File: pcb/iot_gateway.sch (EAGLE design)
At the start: 183 parts, among them CON1 6P-SH-TOP, CON2 6P-SH-TOP, CON3 2P-PH-TOP, J2 DCJACK-SMD, Q1 AO3401, Q2 AO3401, Q3 AO3400, Q4 AO3400, T1 BC817, T2 BC817, T3 BC817, T4 BC817, T5 BC817, U1 EFM32GG11B4XX_Q100, U10 CCS811, U11 MIC4682, U12 MIC4682, U13 MIC39101, U14 FS312F-G, U15 TP4056, U16 FS8205, U17 ER-TFT035-6, U2 SST26VF064B, U3 SST26VF016B, U4 ESP8266EX, U5 RFM69HW, U6 SIM800C, U7 SI7021, U8 SI7210, U9 BMP280, Y1 8 MHz, Y2 32.768 kHz, Y3 24 MHz

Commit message: Update libraries
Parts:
- C24: device Capacitor:CAPACITOR-0603 -> Capacitor:CAPACITOR-1206
- D1: device LED:WS2812B-SMD -> LED:WS2812B-SMD5050
- D4, D5: OCLCSC C129854 -> C129816
- R28, R30, R31, R32, R33: MF VISHAY -> (none)
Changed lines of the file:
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@@
 <?xml version="1.0" encoding="utf-8"?>
 <!DOCTYPE eagle SYSTEM "eagle.dtd">
-<eagle version="9.3.2">
+<eagle version="9.3.0">
 <drawing>
 <settings>
@@
 <part name="GND47" library="Supply Symbol" deviceset="GND" device=""/>
 <part name="R35" library="Resistor" deviceset="RESISTOR" device="-0603" value="0 Ohms"/>
-<part name="C24" library="Capacitor" deviceset="CAPACITOR" device="-0603" value="100uF"/>
+<part name="C24" library="Capacitor" deviceset="CAPACITOR" device="-1206" value="100uF"/>
 <part name="GND42" library="Supply Symbol" deviceset="GND" device=""/>
 <part name="4V23" library="Supply Symbol" deviceset="4V2" device="" value="4V2"/>
@@
 <attribute name="MF" value="FAIRCHILD SEMICONDUCTOR"/>
 </part>
-<part name="R30" library="Resistor" deviceset="RESISTOR" device="-0603" value="330 Ohms">
-<attribute name="MF" value="VISHAY"/>
-</part>
-<part name="R32" library="Resistor" deviceset="RESISTOR" device="-0603" value="10K Ohms">
-<attribute name="MF" value="VISHAY"/>
-</part>
-<part name="R28" library="Resistor" deviceset="RESISTOR" device="-0603" value="10K Ohms">
-<attribute name="MF" value="VISHAY"/>
-</part>
-<part name="R31" library="Resistor" deviceset="RESISTOR" device="-0603" value="10K Ohms">
-<attribute name="MF" value="VISHAY"/>
-</part>
+<part name="R30" library="Resistor" deviceset="RESISTOR" device="-0603" value="330 Ohms"/>
+<part name="R32" library="Resistor" deviceset="RESISTOR" device="-0603" value="10K Ohms"/>
+<part name="R28" library="Resistor" deviceset="RESISTOR" device="-0603" value="10K Ohms"/>
+<part name="R31" library="Resistor" deviceset="RESISTOR" device="-0603" value="10K Ohms"/>
 <part name="D2" library="LED" deviceset="LED" device="1206" value="RED"/>
 <part name="C25" library="Capacitor" deviceset="CAPACITOR" device="-0603" value="1uF"/>
@@
 <attribute name="MF" value="FAIRCHILD SEMICONDUCTOR"/>
 </part>
-<part name="R33" library="Resistor" deviceset="RESISTOR" device="-0603" value="10K Ohms">
-<attribute name="MF" value="VISHAY"/>
-</part>
+<part name="R33" library="Resistor" deviceset="RESISTOR" device="-0603" value="10K Ohms"/>
 <part name="GND46" library="Supply Symbol" deviceset="GND" device=""/>
 <part name="4V24" library="Supply Symbol" deviceset="4V2" device="" value="4V2"/>
@@
 <part name="D6" library="Generic Diode" deviceset="DSK24" device="" value="DSK24"/>
 <part name="D4" library="Generic Diode" deviceset="SK54L" device="" value="SK54L">
-<attribute name="OCLCSC" value="C129854"/>
+<attribute name="OCLCSC" value="C129816"/>
 </part>
 <part name="C32" library="Capacitor" deviceset="CAPACITOR" device="-0603" value="100nF"/>
@@
 <part name="VBAT1" library="Supply Symbol" deviceset="VBAT" device=""/>
 <part name="D5" library="Generic Diode" deviceset="SK54L" device="" value="SK54L">
-<attribute name="OCLCSC" value="C129854"/>
+<attribute name="OCLCSC" value="C129816"/>
 </part>
 <part name="C33" library="Capacitor" deviceset="CAPACITOR" device="-0603" value="100nF"/>
@@
 <part name="GND99" library="Supply Symbol" deviceset="GND" device=""/>
 <part name="J2" library="DC Jack" deviceset="DCJACK" device="-SMD"/>
-<part name="D1" library="LED" deviceset="WS2812B" device="-SMD" value="WS2812B"/>
+<part name="D1" library="LED" deviceset="WS2812B" device="-SMD5050" value="WS2812B"/>
 <part name="GND10" library="Supply Symbol" deviceset="GND" device=""/>
 <part name="C7" library="Capacitor" deviceset="CAPACITOR" device="-0603" value="100nF"/>
@@
 </instance>
 <instance part="R30" gate="G$1" x="96.52" y="157.48" smashed="yes" rot="R90">
-<attribute name="MF" x="96.52" y="157.48" size="1.778" layer="96" rot="R90" display="off"/>
 <attribute name="VALUE" x="100.1776" y="158.1658" size="1.778" layer="96" ratio="10" rot="SR90"/>
 <attribute name="NAME" x="93.7514" y="158.4706" size="1.778" layer="95" ratio="10" rot="SR90"/>
 </instance>
 <instance part="R32" gate="G$1" x="111.76" y="147.32" smashed="yes">
-<attribute name="MF" x="111.76" y="147.32" size="1.778" layer="96" rot="R180" display="off"/>
 <attribute name="VALUE" x="112.4458" y="143.6624" size="1.778" layer="96" ratio="10" rot="SR0"/>
 <attribute name="NAME" x="112.7506" y="150.0886" size="1.778" layer="95" ratio="10" rot="SR0"/>
 </instance>
 <instance part="R28" gate="G$1" x="73.66" y="114.3" smashed="yes">
-<attribute name="MF" x="73.66" y="114.3" size="1.778" layer="96" rot="R180" display="off"/>
 <attribute name="VALUE" x="74.3458" y="110.6424" size="1.778" layer="96" ratio="10" rot="SR0"/>
 <attribute name="NAME" x="74.6506" y="117.0686" size="1.778" layer="95" ratio="10" rot="SR0"/>
 </instance>
 <instance part="R31" gate="G$1" x="106.68" y="142.24" smashed="yes" rot="R270">
-<attribute name="MF" x="106.68" y="142.24" size="1.778" layer="96" rot="R90" display="off"/>
 <attribute name="VALUE" x="103.0224" y="141.5542" size="1.778" layer="96" ratio="10" rot="SR270"/>
 <attribute name="NAME" x="109.4486" y="141.2494" size="1.778" layer="95" ratio="10" rot="SR270"/>
@@
 </instance>
 <instance part="R33" gate="G$1" x="147.32" y="177.8" smashed="yes">
-<attribute name="MF" x="147.32" y="177.8" size="1.778" layer="96" rot="R180" display="off"/>
 <attribute name="VALUE" x="148.0058" y="174.1424" size="1.778" layer="96" ratio="10" rot="SR0"/>
 <attribute name="NAME" x="148.3106" y="180.5686" size="1.778" layer="95" ratio="10" rot="SR0"/>

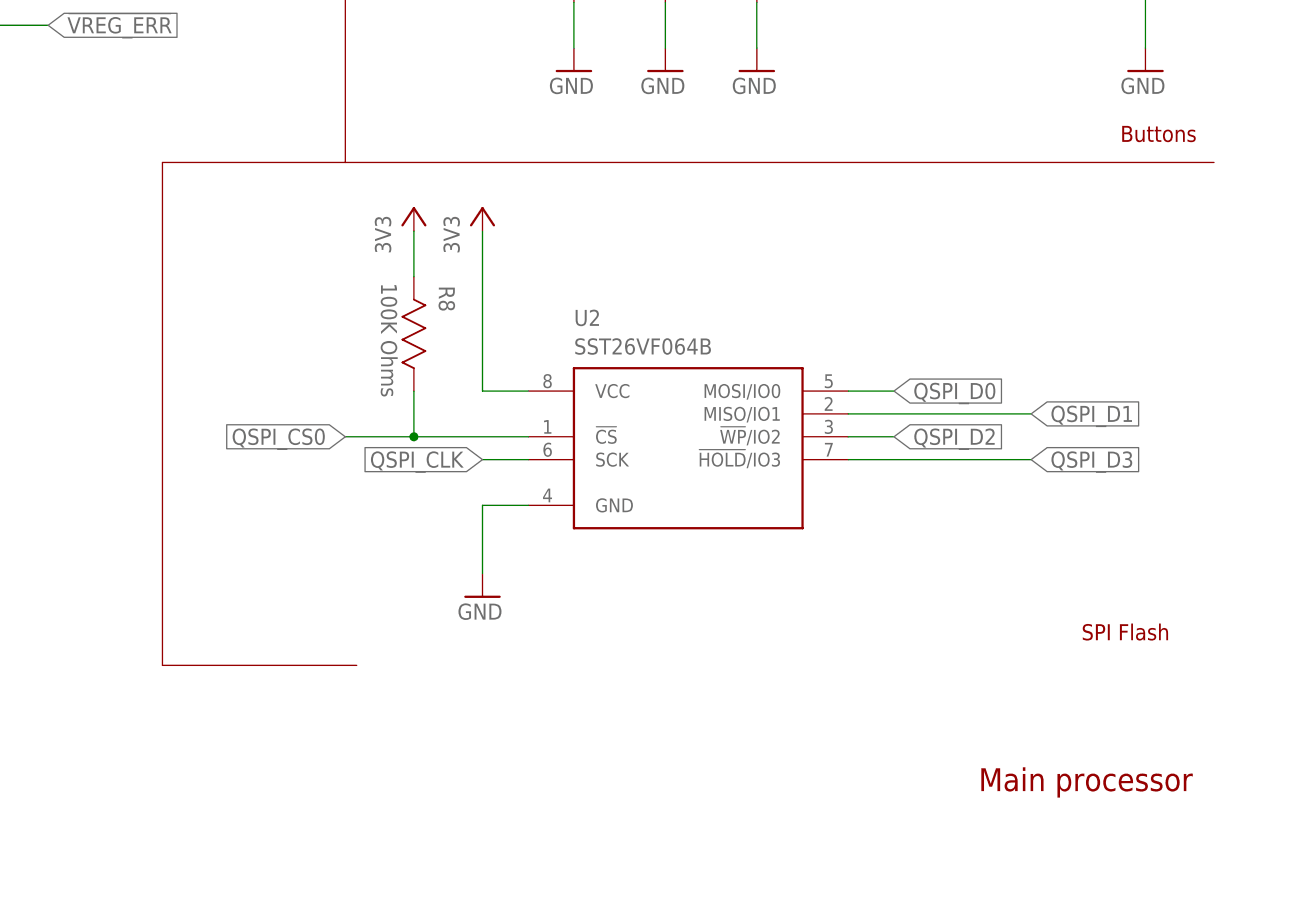
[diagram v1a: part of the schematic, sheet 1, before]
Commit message: Final board ordered
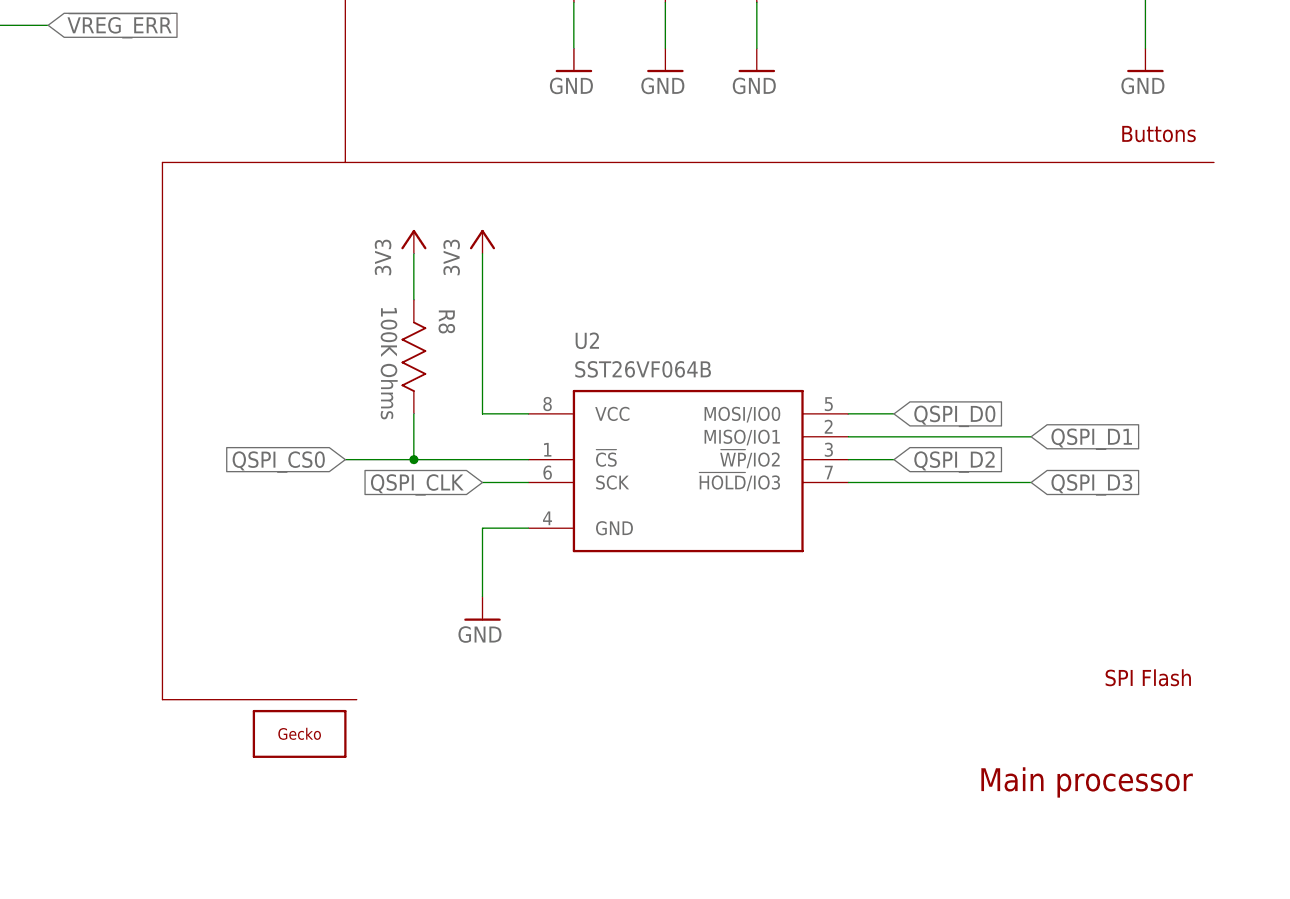
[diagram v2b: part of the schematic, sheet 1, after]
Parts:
- added U$1: GECKO, Silkscreen:GECKO
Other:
- moved on the sheet: R8, U2
